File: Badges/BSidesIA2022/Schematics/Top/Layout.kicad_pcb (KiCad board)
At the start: 2 copper layers, 69.9 x 139.7 mm, 7 parts

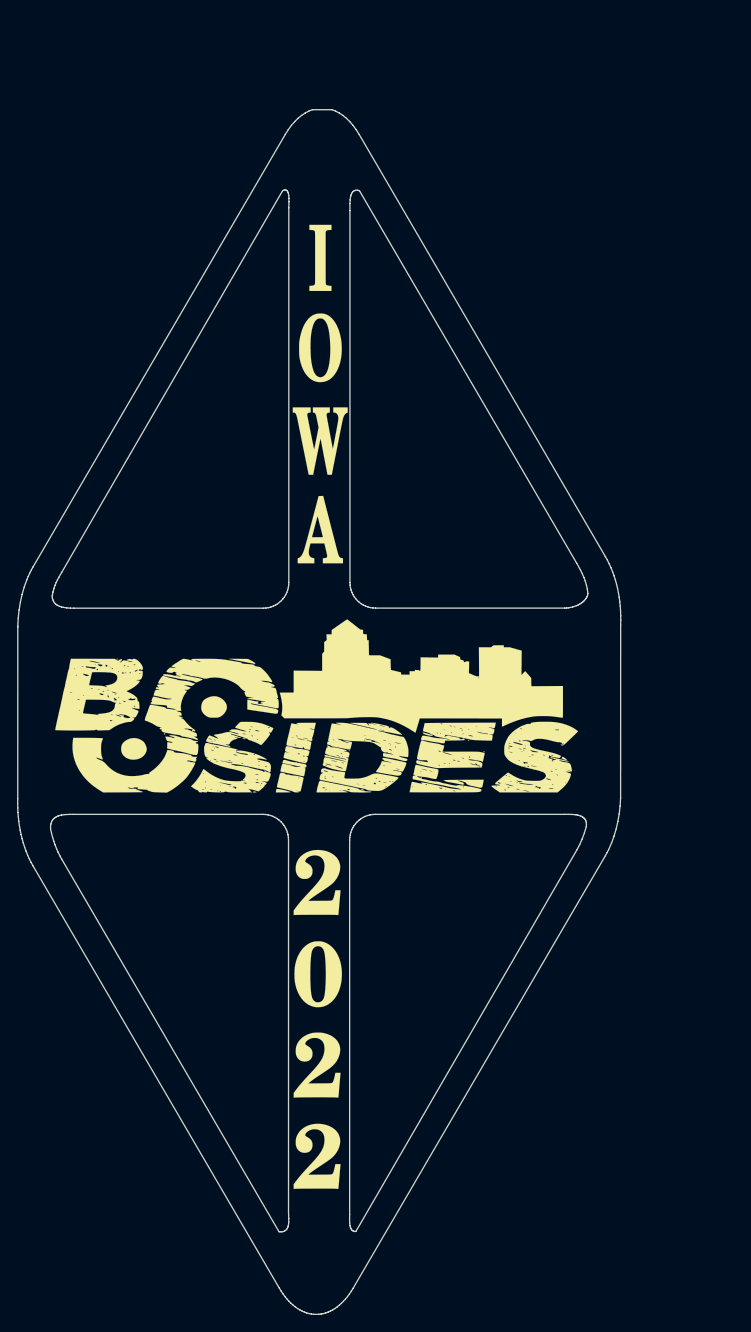
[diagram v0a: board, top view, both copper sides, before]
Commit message: Mostly final Corncon
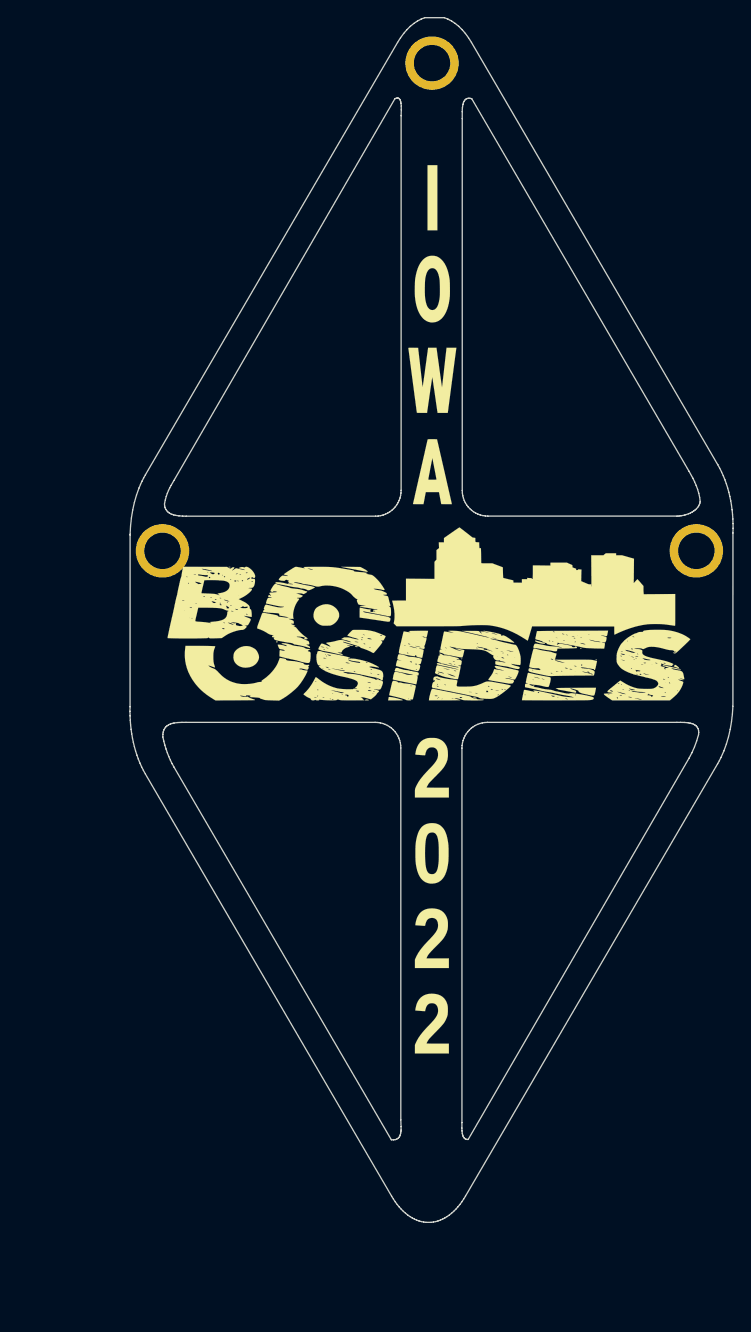
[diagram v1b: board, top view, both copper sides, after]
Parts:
- removed the G*** at (136.9, 122.3) (x4)
- added G*** (x4): LOGO, LOGO, F.Cu at (149.9, 111.7)
- added H1: MountingHole, cafebabe:SMD Spacer M2.5, F.Cu at (177.2, 90.5)
- added H2: MountingHole, cafebabe:SMD Spacer M2.5, F.Cu at (115.3, 90.5)
- added H3: MountingHole, cafebabe:SMD Spacer M2.5, F.Cu at (146.6, 33.9)
- moved G*** 16.8 mm to (149.9, 111.7) (x3)
